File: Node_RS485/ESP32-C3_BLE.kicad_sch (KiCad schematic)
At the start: 30 parts, among them J4 CONN_ESP_PROG, J5 USB_C_Receptacle_USB2.0_16P, Q2 SI2301, SW2 ESP-RESET, SW3 ESP-BOOT, U10 USBLC6-2SC6, U9 ESP32-C3, Y1 40MHz

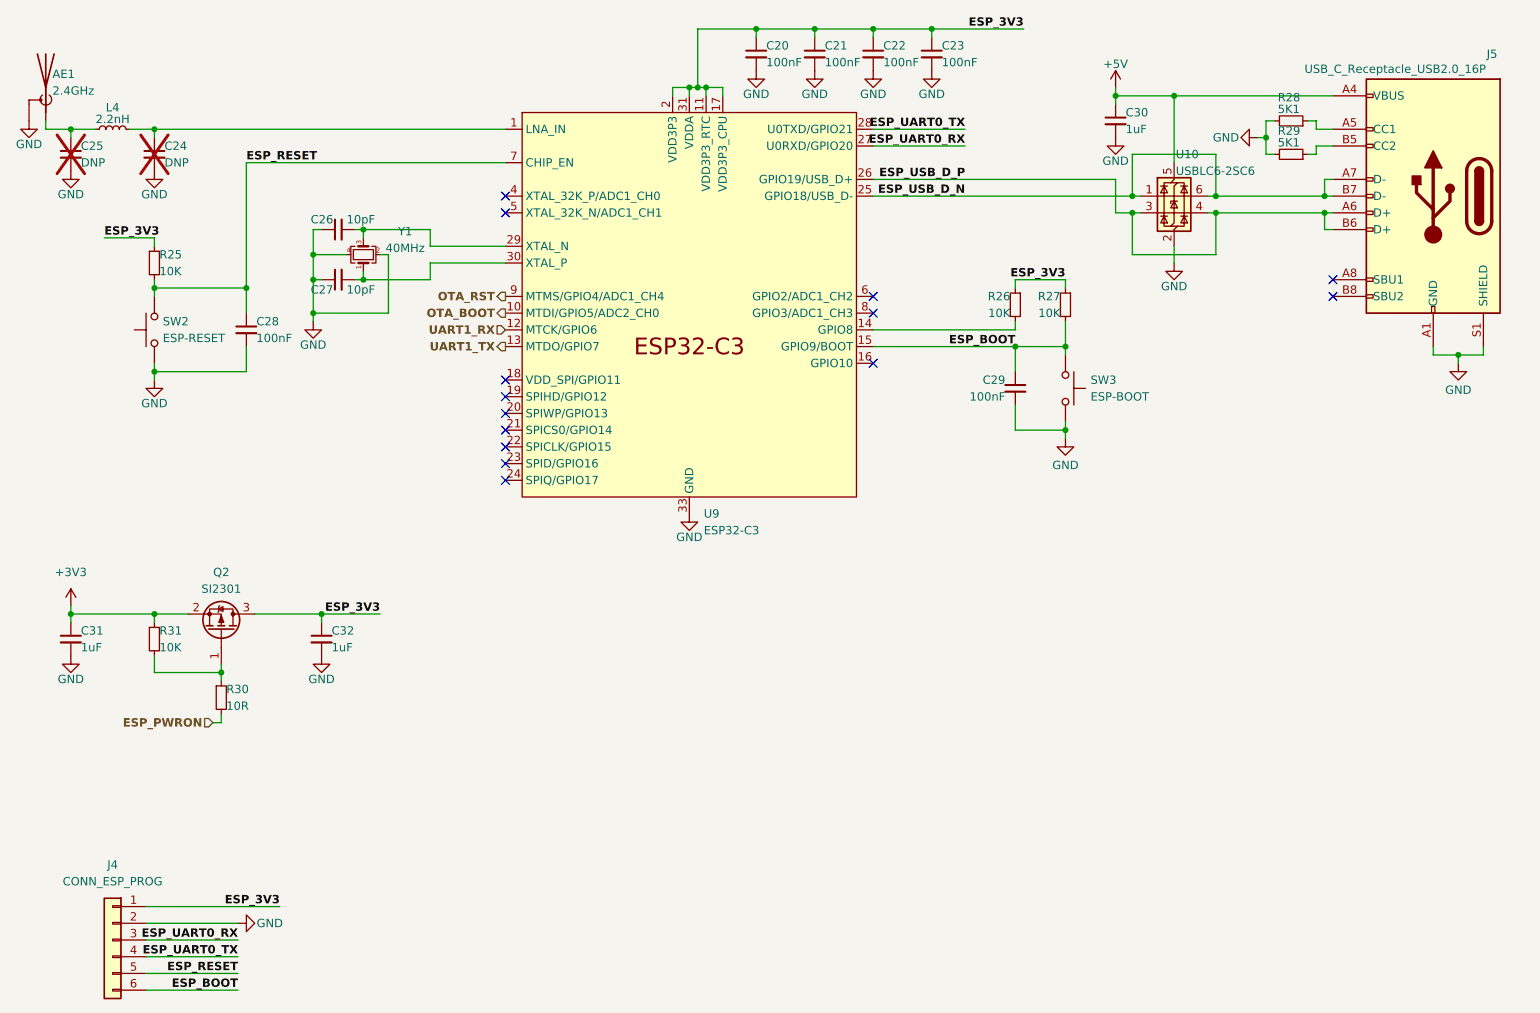
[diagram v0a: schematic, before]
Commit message: New version.
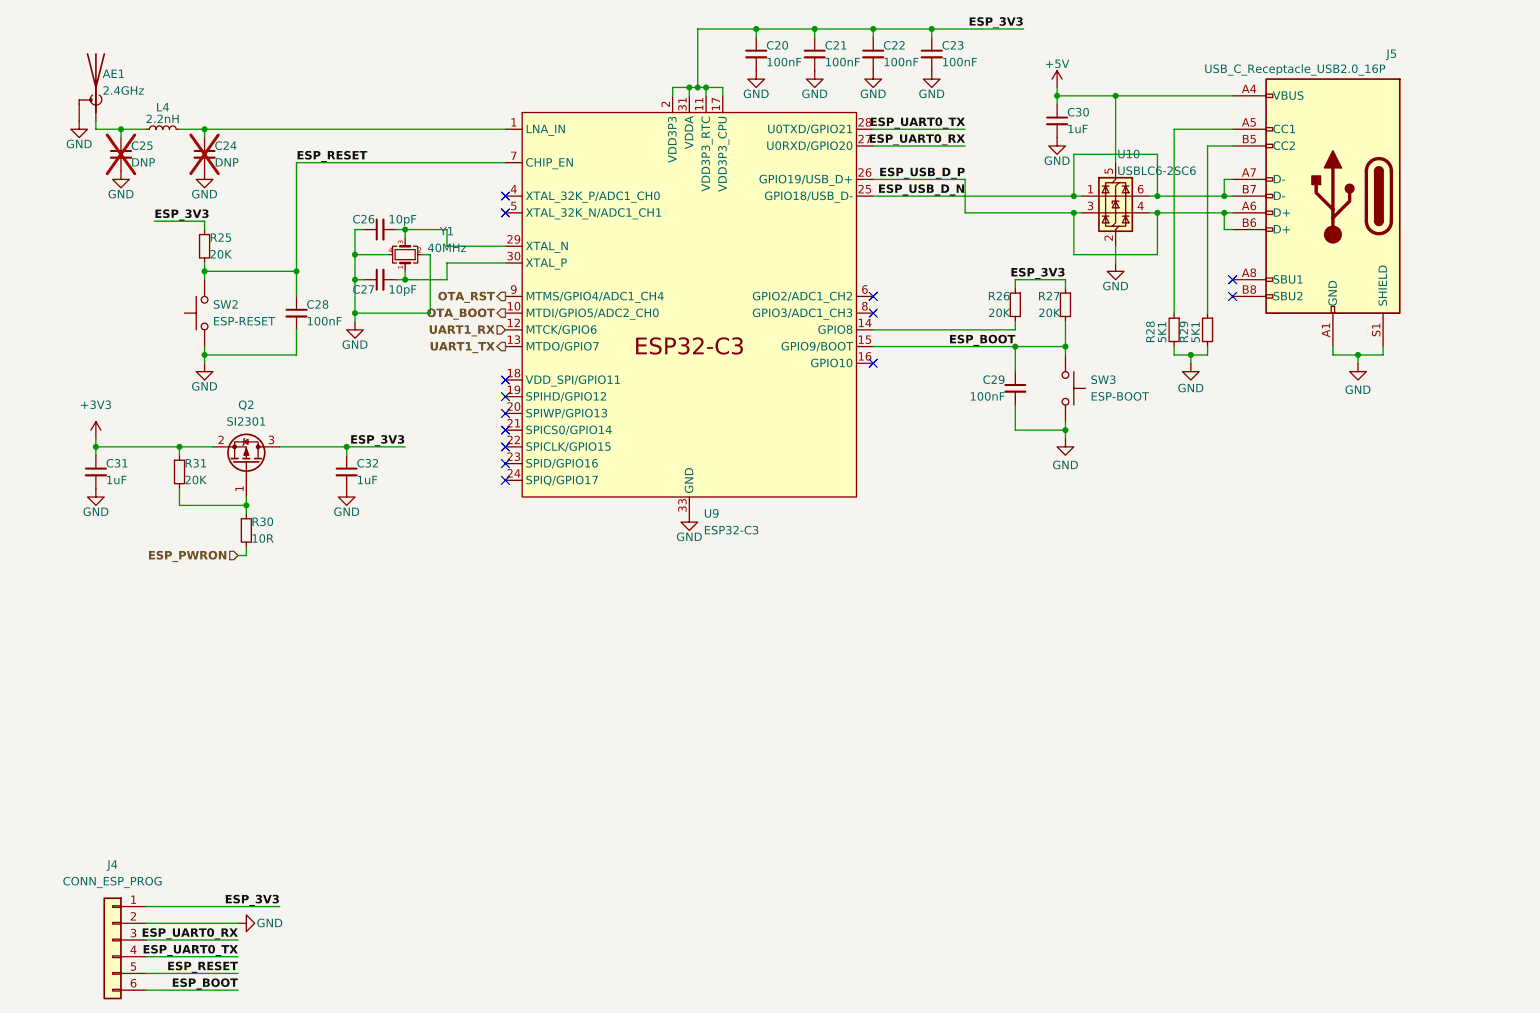
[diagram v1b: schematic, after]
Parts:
- R25, R26, R27, R31: value 10K -> 20K
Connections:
- net ESP_USB_D_P is gone; now on net ESP_USB_D_N: J5.A6 (D+), J5.B6 (D+), U10.3 (I/O2), U10.4 (I/O2), U9.26 (GPIO19/USB_D+)
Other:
- moved on the sheet: AE1, C24, C25, C26, C27, C28, C30, C31, C32, J5, L4, Q2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
